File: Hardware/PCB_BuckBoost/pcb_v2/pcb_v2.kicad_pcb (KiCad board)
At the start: 2 copper layers, 43 x 69 mm, 42 parts, among them J1 Conn_01x02, J2 Conn_01x02, J3 Conn_01x02, J4 Conn_01x02, U1 MIC3172YM, U2 MIC3172YM

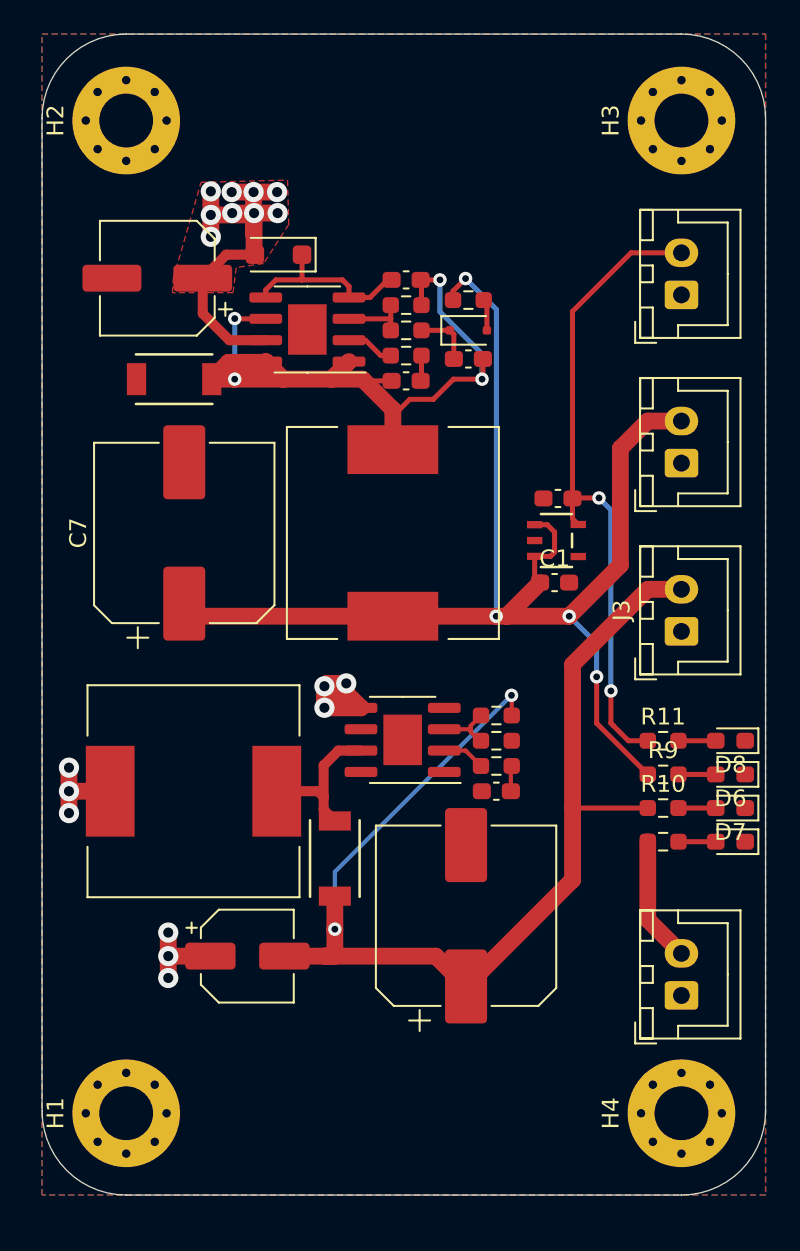
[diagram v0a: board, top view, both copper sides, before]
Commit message: PCB V3 VRAIMENT FINI
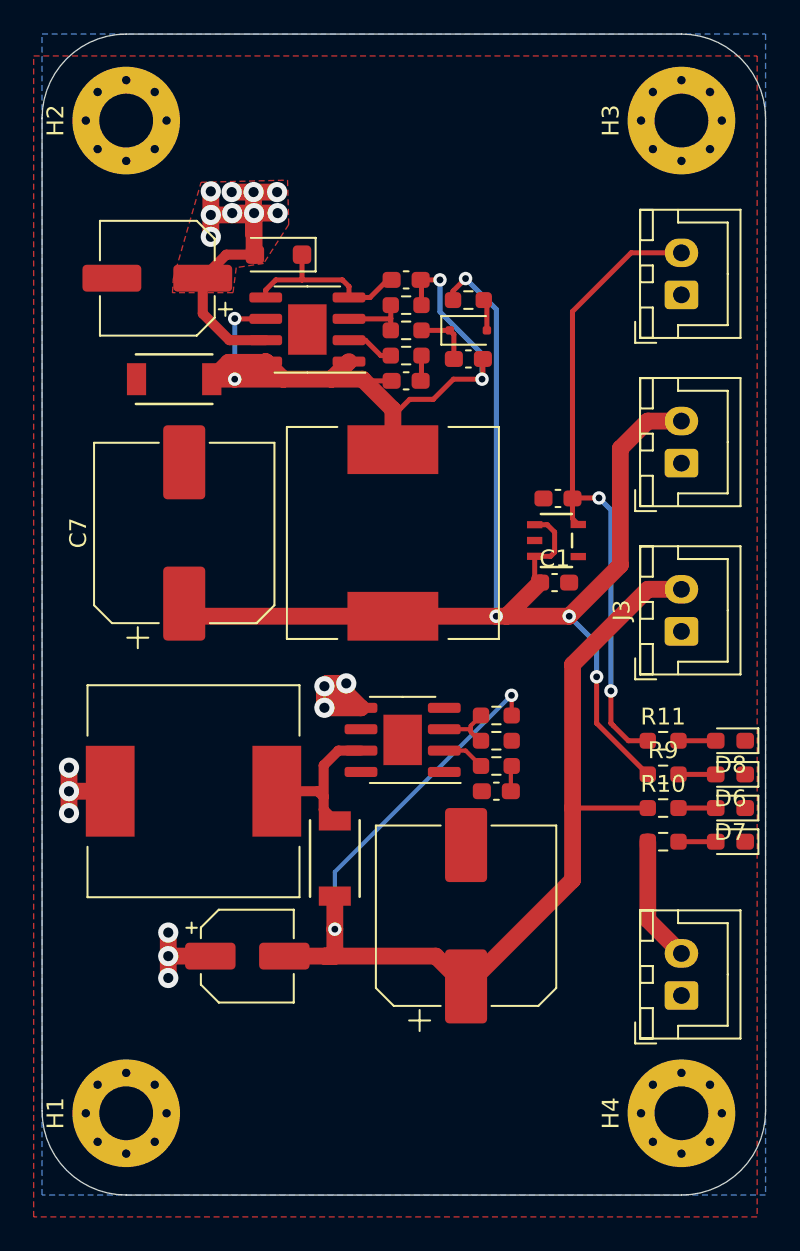
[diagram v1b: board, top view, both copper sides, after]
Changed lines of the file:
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@@
     (polygon
       (pts
-        (xy 173.5 120.7)
-        (xy 173.5 51.7)
-        (xy 216.5 51.7)
-        (xy 216.5 120.7)
+        (xy 173 122)
+        (xy 173 53)
+        (xy 216 53)
+        (xy 216 122)
       )
     )
